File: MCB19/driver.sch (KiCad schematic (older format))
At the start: 26 parts, among them J611 +BATT, J612 GND, J613 VBAT+, J614 VBAT-, Q601 IRFP260N, Q602 IRFP260N, U601 LM5104MNOPB, U602 INA211_DCK_6, U603 LM324

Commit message: Novos detalhes na placa
Comecei a planejar onde ficam os componentes da placa, em especial os que fazem parte do buck e os que estão no atmega328p, exceto os do driver
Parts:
- U601: symbol INA211BIDCKR:LM5104MNOPB -> MCB19-rescue:LM5104MNOPB-INA211BIDCKR
- U602: symbol INA211BIDCKR:INA211_DCK_6 -> MCB19-rescue:INA211_DCK_6-INA211BIDCKR
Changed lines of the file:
@@
 EESchema Schematic File Version 4
 LIBS:MCB19-cache
-EELAYER 26 0
+EELAYER 29 0
 EELAYER END
 $Descr A4 11693 8268
@@
 Connection ~ 6150 2775
 $Comp
-L INA211BIDCKR:INA211_DCK_6 U602
+L MCB19-rescue:INA211_DCK_6-INA211BIDCKR U602
 U 1 1 5D42E6BA
 P 6625 2275
@@
 IRALLL
 $Comp
-L INA211BIDCKR:LM5104MNOPB U601
+L MCB19-rescue:LM5104MNOPB-INA211BIDCKR U601
 U 1 1 5D437554
 P 2375 3850

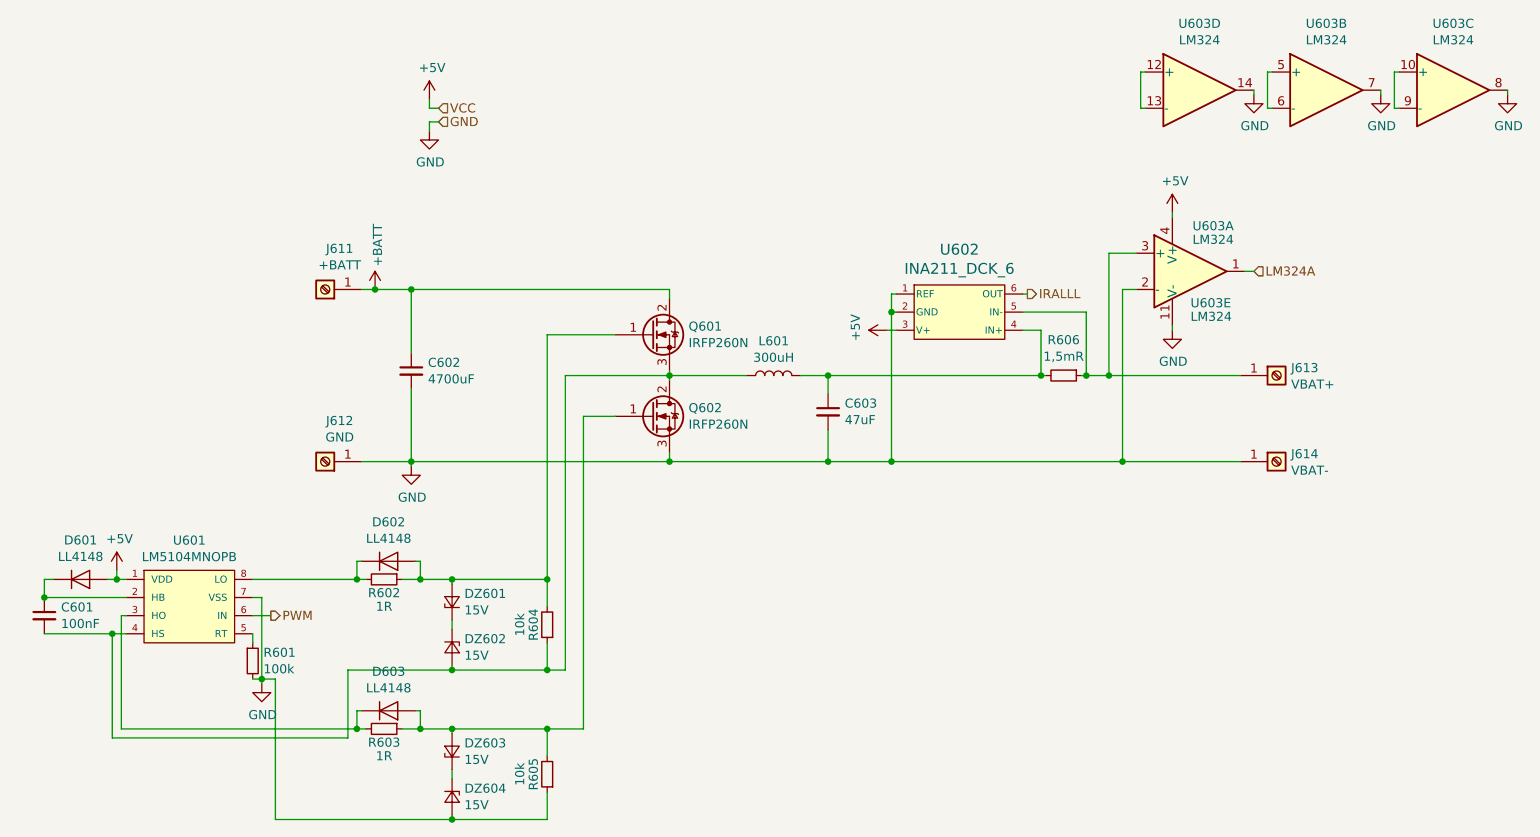
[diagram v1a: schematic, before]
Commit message: Add files via upload
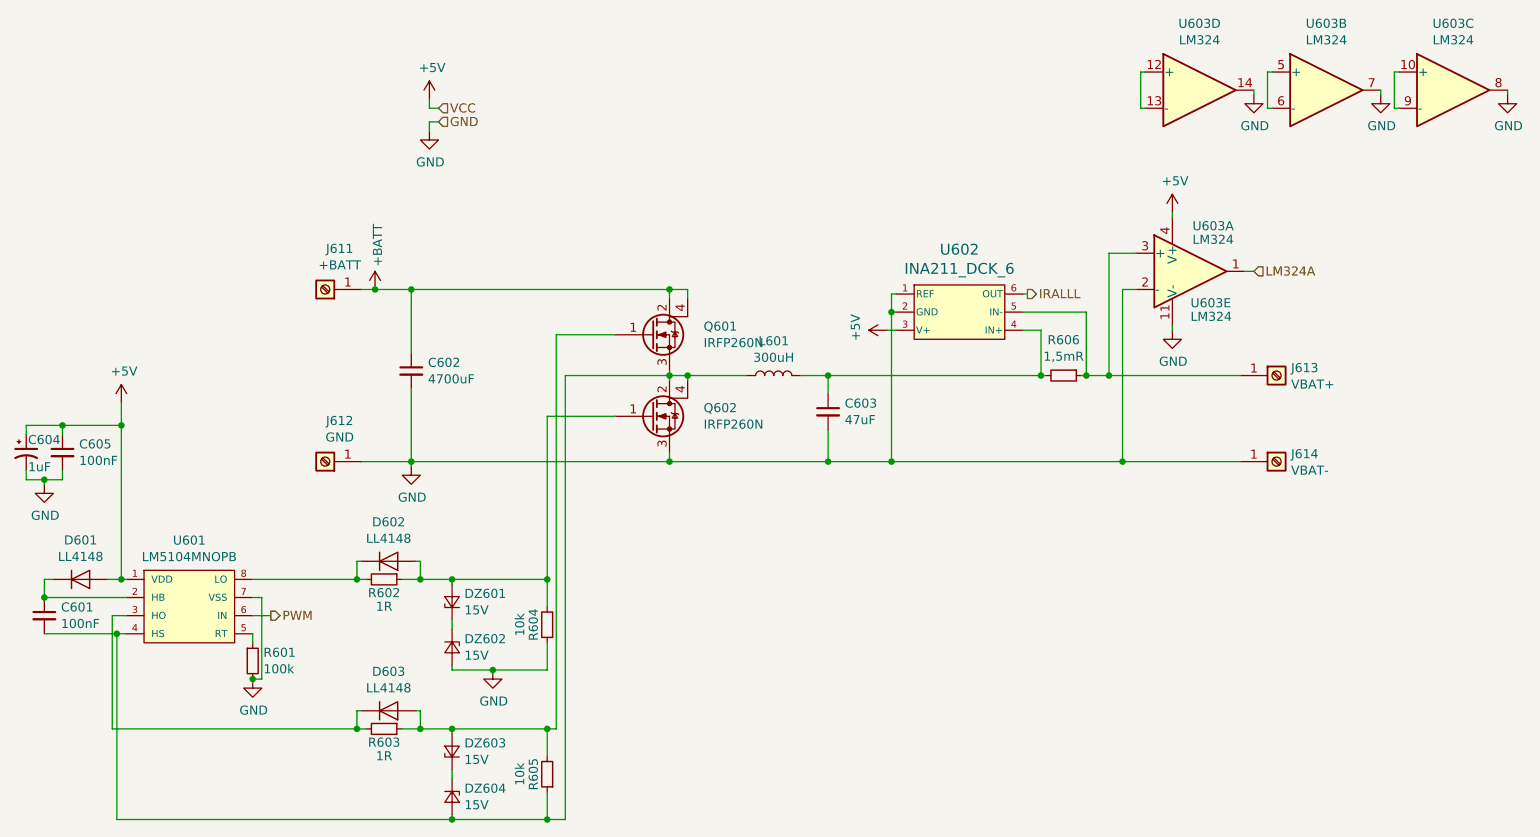
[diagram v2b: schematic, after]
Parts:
- removed Q601, Q602: IRFP260N, KicadZeniteSolarLibrary18:TO-247-3_Horizontal_TabDown_SMD, symbol Device:Q_NMOS_GDS
- added C604: 1uF, Capacitor_Tantalum_SMD:CP_EIA-6032-20_AVX-F_Pad2.25x2.35mm_HandSolder, symbol Device:CP1_Small
- added C605: 100nF, Capacitor_SMD:C_0805_2012Metric_Pad1.15x1.40mm_HandSolder, symbol Device:C_Small
- added Q601, Q602: IRFP260N, KicadZeniteSolarLibrary18:TO-247-3_Horizontal_TabDown_SMD, symbol Device:Q_NMOS_GDSD
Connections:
- net +5V: now also C604.1, C605.1
- net +BATT: now also Q601.2 (D), Q601.4 (D)
- net GND: now also DZ602.2 (A), R604.1, C604.2, C605.2, Q602.3 (S); no longer DZ604.2 (A), R605.1
- net at D602.2 (A), DZ601.2 (A), R602.1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: now also Q602.1 (G)
- net at C601.2, L601.1, U601.4 (HS): now also DZ604.2 (A), R605.1, Q601.3 (S), Q602.2 (D), Q602.4 (D); no longer DZ602.2 (A), R604.1
- net at D603.2 (A), DZ603.2 (A), R603.1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: now also Q601.1 (G)
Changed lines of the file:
@@
 Wire Wire Line
 	3850 2300 3850 2650
-$Comp
-L Device:Q_NMOS_GDS Q601
-U 1 1 5D42B3E2
-P 5175 2550
-F 0 "Q601" H 5380 2596 50  0000 L CNN
-F 1 "IRFP260N" H 5380 2505 50  0000 L CNN
-F 2 "KicadZeniteSolarLibrary18:TO-247-3_Horizontal_TabDown_SMD" H 5375 2650 50  0001 C CNN
-F 3 "~" H 5175 2550 50  0001 C CNN
-	1    5175 2550
-	1    0    0    -1
-$EndComp
-$Comp
-L Device:Q_NMOS_GDS Q602
-U 1 1 5D42B435
-P 5175 3000
-F 0 "Q602" H 5380 3046 50  0000 L CNN
-F 1 "IRFP260N" H 5380 2955 50  0000 L CNN
-F 2 "KicadZeniteSolarLibrary18:TO-247-3_Horizontal_TabDown_SMD" H 5375 3100 50  0001 C CNN
-F 3 "~" H 5175 3000 50  0001 C CNN
-	1    5175 3000
-	1    0    0    -1
-$EndComp
 Wire Wire Line
 	5275 2750 5275 2775
@@
 $EndComp
 Wire Wire Line
-	5275 2775 5700 2775
+	5275 2775 5375 2775
 Connection ~ 5275 2775
 Wire Wire Line
@@
 IRALLL
 $Comp
-L MCB19-rescue:LM5104MNOPB-INA211BIDCKR U601
-U 1 1 5D437554
-P 2375 3850
-F 0 "U601" H 2625 4015 50  0000 C CNN
-F 1 "LM5104MNOPB" H 2625 3924 50  0000 C CNN
-F 2 "Package_SO:SOIC-8_3.9x4.9mm_P1.27mm" H 2375 3850 50  0001 C CNN
-F 3 "" H 2375 3850 50  0001 C CNN
-	1    2375 3850
-	1    0    0    -1
-$EndComp
-$Comp
 L power:+5V #PWR0109
 U 1 1 5D438678
-P 2225 3850
-F 0 "#PWR0109" H 2225 3700 50  0001 C CNN
-F 1 "+5V" H 2240 4023 50  0000 C CNN
-F 2 "" H 2225 3850 50  0001 C CNN
-F 3 "" H 2225 3850 50  0001 C CNN
-	1    2225 3850
-	1    0    0    -1
-$EndComp
-Wire Wire Line
-	2275 3900 2225 3900
-Wire Wire Line
-	2225 3900 2225 3850
-$Comp
-L power:GND #PWR0108
-U 1 1 5D438BD1
-P 3025 4475
-F 0 "#PWR0108" H 3025 4225 50  0001 C CNN
-F 1 "GND" H 3030 4302 50  0000 C CNN
-F 2 "" H 3025 4475 50  0001 C CNN
-F 3 "" H 3025 4475 50  0001 C CNN
-	1    3025 4475
-	1    0    0    -1
-$EndComp
+P 2250 2925
+F 0 "#PWR0109" H 2250 2775 50  0001 C CNN
+F 1 "+5V" H 2265 3098 50  0000 C CNN
+F 2 "" H 2250 2925 50  0001 C CNN
+F 3 "" H 2250 2925 50  0001 C CNN
+	1    2250 2925
+	1    0    0    -1
+$EndComp
+Wire Wire Line
+	2275 3900 2250 3900
 Wire Wire Line
 	2975 4000 3025 4000
@@
 $EndComp
 Wire Wire Line
-	2225 3900 2175 3900
-Connection ~ 2225 3900
-Wire Wire Line
 	1875 3900 1825 3900
 Wire Wire Line
@@
 Wire Wire Line
 	2975 4450 3025 4450
-Connection ~ 3025 4450
-Wire Wire Line
-	3025 4450 3025 4475
 $Comp
 L Device:C_Small C601
@@
 $EndComp
 Connection ~ 1825 4000
-Wire Wire Line
-	1825 4200 2200 4200
 $Comp
 L Device:R_Small R602
@@
 $EndComp
 Wire Wire Line
-	2275 4100 2250 4100
-Wire Wire Line
-	2250 4100 2250 4725
-Wire Wire Line
 	2975 3900 3550 3900
 $Comp
@@
 	1    0    0    1
 $EndComp
-Wire Wire Line
-	2250 4725 3550 4725
 $Comp
 L Diode:LL4148 D602
@@
 	4075 4375 4075 4400
 Wire Wire Line
-	4075 4400 4600 4400
+	4075 4400 4300 4400
 Wire Wire Line
 	4600 4400 4600 4250
@@
 	4600 3900 4075 3900
 Connection ~ 4075 3900
-Wire Wire Line
-	2200 4200 2200 4775
-Wire Wire Line
-	2200 4775 3500 4775
-Wire Wire Line
-	3500 4775 3500 4400
-Wire Wire Line
-	3500 4400 4075 4400
-Connection ~ 2200 4200
-Wire Wire Line
-	2200 4200 2275 4200
-Connection ~ 4075 4400
 Connection ~ 3900 3900
 $Comp
@@
 	4075 5200 4075 5225
 Wire Wire Line
-	4075 5225 4600 5225
-Wire Wire Line
 	4600 5225 4600 5075
 Wire Wire Line
@@
 	4600 4725 4075 4725
 Connection ~ 4075 4725
-Connection ~ 4075 5225
-Wire Wire Line
-	3025 4450 3100 4450
-Wire Wire Line
-	3100 4450 3100 5225
-Wire Wire Line
-	3100 5225 4075 5225
 Connection ~ 3900 4725
-Wire Wire Line
-	4600 3900 4600 2550
-Wire Wire Line
-	4600 2550 4975 2550
-Connection ~ 4600 3900
 Connection ~ 4600 4725
 $Comp
@@
 	7775 3250 8425 3250
 Wire Wire Line
-	4600 4400 4700 4400
-Connection ~ 4600 4400
-Wire Wire Line
-	4700 2775 5275 2775
-Wire Wire Line
-	4700 2775 4700 4400
-Wire Wire Line
-	4975 3000 4800 3000
-Wire Wire Line
-	4800 3000 4800 4725
-Wire Wire Line
-	4600 4725 4800 4725
+	4600 4725 4650 4725
 $Comp
 L Connector:Screw_Terminal_01x01 J611
@@
 	-1   0    0    1
 $EndComp
+$Comp
+L Device:Q_NMOS_GDSD Q601
+U 1 1 5D4779AA
+P 5175 2550
+F 0 "Q601" H 5463 2596 50  0000 L CNN
+F 1 "IRFP260N" H 5463 2505 50  0000 L CNN
+F 2 "KicadZeniteSolarLibrary18:TO-247-3_Horizontal_TabDown_SMD" H 5375 2650 50  0001 C CNN
+F 3 "~" H 5175 2550 50  0001 C CNN
+	1    5175 2550
+	1    0    0    -1
+$EndComp
+$Comp
+L Device:Q_NMOS_GDSD Q602
+U 1 1 5D479074
+P 5175 3000
+F 0 "Q602" H 5463 3046 50  0000 L CNN
+F 1 "IRFP260N" H 5463 2955 50  0000 L CNN
+F 2 "KicadZeniteSolarLibrary18:TO-247-3_Horizontal_TabDown_SMD" H 5375 3100 50  0001 C CNN
+F 3 "~" H 5175 3000 50  0001 C CNN
+	1    5175 3000
+	1    0    0    -1
+$EndComp
+Wire Wire Line
+	5375 2350 5375 2300
+Wire Wire Line
+	5375 2300 5275 2300
+Connection ~ 5275 2300
+Wire Wire Line
+	5375 2800 5375 2775
+Connection ~ 5375 2775
+Wire Wire Line
+	5375 2775 5700 2775
+$Comp
+L Device:CP1_Small C?
+U 1 1 5D47B02C
+P 1725 3200
+AR Path="/5AACFFEF/5D47B02C" Ref="C?"  Part="1"
+AR Path="/5D414D87/5D47B02C" Ref="C604"  Part="1"
+F 0 "C604" H 1735 3270 50  0000 L CNN
+F 1 "1uF" H 1735 3120 50  0000 L CNN
+F 2 "Capacitor_Tantalum_SMD:CP_EIA-6032-20_AVX-F_Pad2.25x2.35mm_HandSolder" H 1725 3200 50  0001 C CNN
+F 3 "" H 1725 3200 50  0001 C CNN
+	1    1725 3200
+	1    0    0    -1
+$EndComp
+$Comp
+L Device:C_Small C605
+U 1 1 5D480B54
+P 1925 3200
+F 0 "C605" H 2017 3246 50  0000 L CNN
+F 1 "100nF" H 2017 3155 50  0000 L CNN
+F 2 "Capacitor_SMD:C_0805_2012Metric_Pad1.15x1.40mm_HandSolder" H 1925 3200 50  0001 C CNN
+F 3 "~" H 1925 3200 50  0001 C CNN
+	1    1925 3200
+	1    0    0    -1
+$EndComp
+Wire Wire Line
+	1725 3300 1725 3350
+Wire Wire Line
+	1725 3350 1825 3350
+Wire Wire Line
+	1925 3350 1925 3300
+Wire Wire Line
+	1725 3100 1725 3050
+Wire Wire Line
+	1925 3050 1925 3100
+Wire Wire Line
+	2250 3050 2250 2925
+Wire Wire Line
+	1725 3050 1925 3050
+Connection ~ 1925 3050
+Wire Wire Line
+	1925 3050 2250 3050
+Wire Wire Line
+	2250 3050 2250 3900
+Connection ~ 2250 3050
+Connection ~ 2250 3900
+Wire Wire Line
+	2175 3900 2250 3900
+$Comp
+L MCB19-rescue:LM5104MNOPB-INA211BIDCKR U601
+U 1 1 5D437554
+P 2375 3850
+F 0 "U601" H 2625 4015 50  0000 C CNN
+F 1 "LM5104MNOPB" H 2625 3924 50  0000 C CNN
+F 2 "Package_SO:SOIC-8_3.9x4.9mm_P1.27mm" H 2375 3850 50  0001 C CNN
+F 3 "" H 2375 3850 50  0001 C CNN
+	1    2375 3850
+	1    0    0    -1
+$EndComp
+$Comp
+L power:GND #PWR0108
+U 1 1 5D438BD1
+P 2975 4450
+F 0 "#PWR0108" H 2975 4200 50  0001 C CNN
+F 1 "GND" H 2980 4277 50  0000 C CNN
+F 2 "" H 2975 4450 50  0001 C CNN
+F 3 "" H 2975 4450 50  0001 C CNN
+	1    2975 4450
+	1    0    0    -1
+$EndComp
+$Comp
+L power:GND #PWR0110
+U 1 1 5D4A1ABA
+P 1825 3375
+F 0 "#PWR0110" H 1825 3125 50  0001 C CNN
+F 1 "GND" H 1830 3202 50  0000 C CNN
+F 2 "" H 1825 3375 50  0001 C CNN
+F 3 "" H 1825 3375 50  0001 C CNN
+	1    1825 3375
+	1    0    0    -1
+$EndComp
+Wire Wire Line
+	1825 3350 1825 3375
+Connection ~ 1825 3350
+Wire Wire Line
+	1825 3350 1925 3350
+Connection ~ 4075 5225
+Connection ~ 4600 3900
+Wire Wire Line
+	4600 3900 4600 3000
+Connection ~ 2975 4450
+Wire Wire Line
+	1825 4200 2225 4200
+Wire Wire Line
+	2200 4100 2200 4725
+Wire Wire Line
+	2200 4100 2275 4100
+Wire Wire Line
+	2225 4200 2225 5225
+Connection ~ 2225 4200
+Wire Wire Line
+	2225 4200 2275 4200
+Wire Wire Line
+	2200 4725 3550 4725
+Wire Wire Line
+	2225 5225 4075 5225
+$Comp
+L power:GND #PWR0111
+U 1 1 5D4C842A
+P 4300 4400
+F 0 "#PWR0111" H 4300 4150 50  0001 C CNN
+F 1 "GND" H 4305 4227 50  0000 C CNN
+F 2 "" H 4300 4400 50  0001 C CNN
+F 3 "" H 4300 4400 50  0001 C CNN
+	1    4300 4400
+	1    0    0    -1
+$EndComp
+Connection ~ 4300 4400
+Wire Wire Line
+	4300 4400 4600 4400
+Wire Wire Line
+	4600 3000 4975 3000
+Wire Wire Line
+	4650 2550 4650 4725
+Wire Wire Line
+	4700 5225 4700 2775
+Wire Wire Line
+	4075 5225 4600 5225
+Connection ~ 4600 5225
+Wire Wire Line
+	4600 5225 4700 5225
+Wire Wire Line
+	4700 2775 5275 2775
+Wire Wire Line
+	4650 2550 4975 2550
 $EndSCHEMATC

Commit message: Final
Design de layout pronto
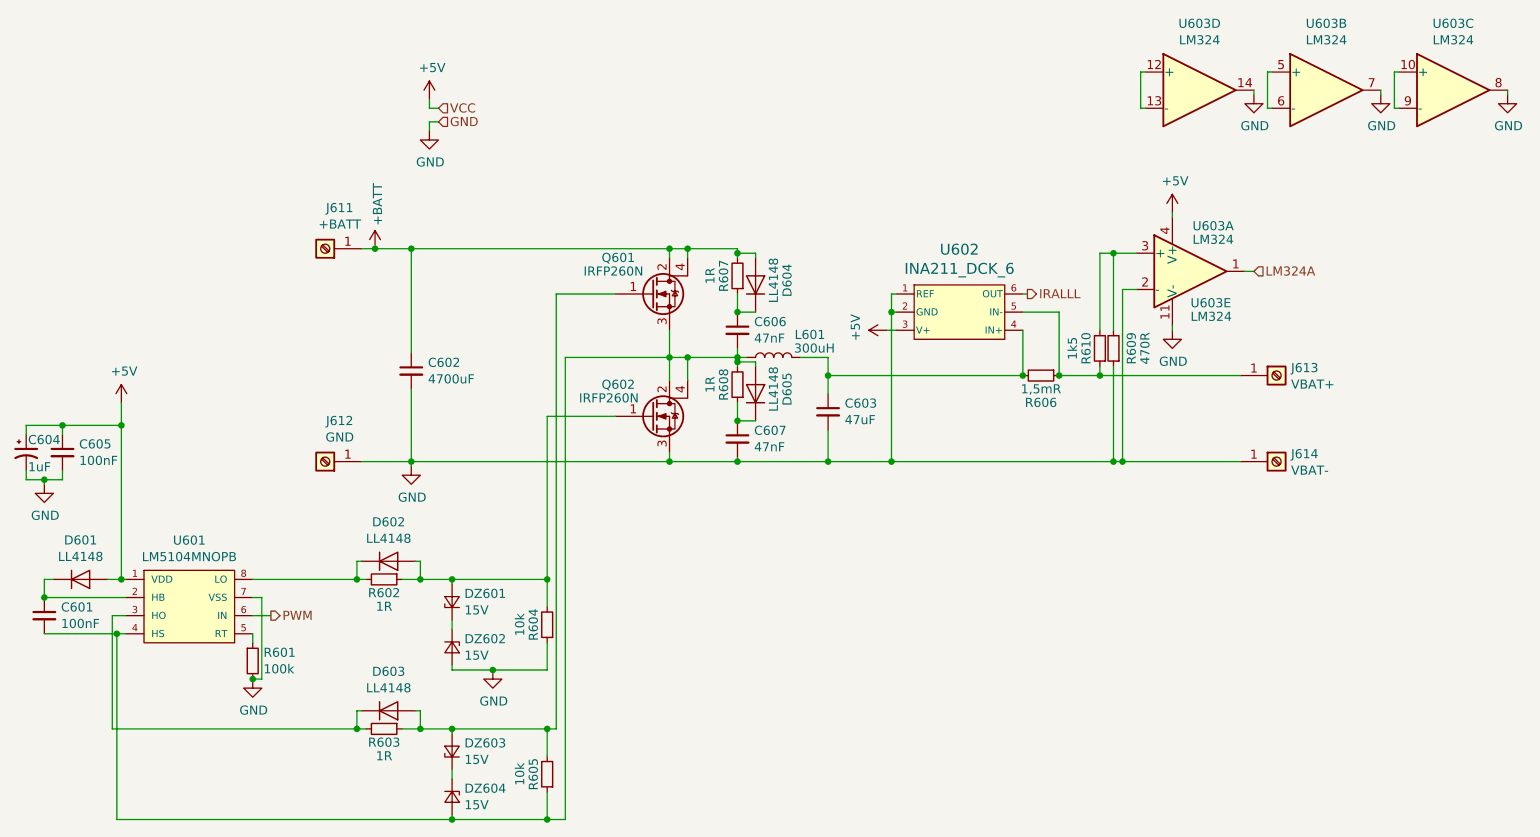
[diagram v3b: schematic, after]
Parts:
- added C606, C607: 47nF, Capacitor_SMD:C_0805_2012Metric_Pad1.15x1.40mm_HandSolder, symbol Device:C_Small
- added D604, D605: LL4148, Diode_SMD:D_MiniMELF_Handsoldering, symbol Diode:LL4148
- added R607, R608: 1R, Resistor_SMD:R_0805_2012Metric_Pad1.15x1.40mm_HandSolder, symbol Device:R_Small
- added R609: 470R, Resistor_SMD:R_0805_2012Metric_Pad1.15x1.40mm_HandSolder, symbol Device:R_Small
- added R610: 1k5, Resistor_SMD:R_0805_2012Metric_Pad1.15x1.40mm_HandSolder, symbol Device:R_Small
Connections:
- net +BATT: now also D604.2 (A), R607.2
- net GND: now also C607.2, R609.1
- net at C601.2, DZ604.2 (A), L601.1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: now also C606.2, D605.2 (A), R608.2
- net at J613.1 (Pin_1), R606.1, U602.5 (IN-): now also R610.1; no longer U603.3 (+)
- new net: R609.2, R610.2, U603.3 (+)
- new net: C606.1, D604.1 (K), R607.1
- new net: C607.1, D605.1 (K), R608.1
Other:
- moved on the sheet: J611, L601, Q601, R606
